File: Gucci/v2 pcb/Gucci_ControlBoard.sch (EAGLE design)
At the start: 70 parts, among them U1 PCA9306_LSSOP, U2 TEENSY_3.6_DIL, U3 MAX4173-SOT-23, U4 MAX4173-SOT-23, U5 LM393-8-SOIC, U6 AP2114H-1.8TRG1, U7 AP2114H-3.3TRG1

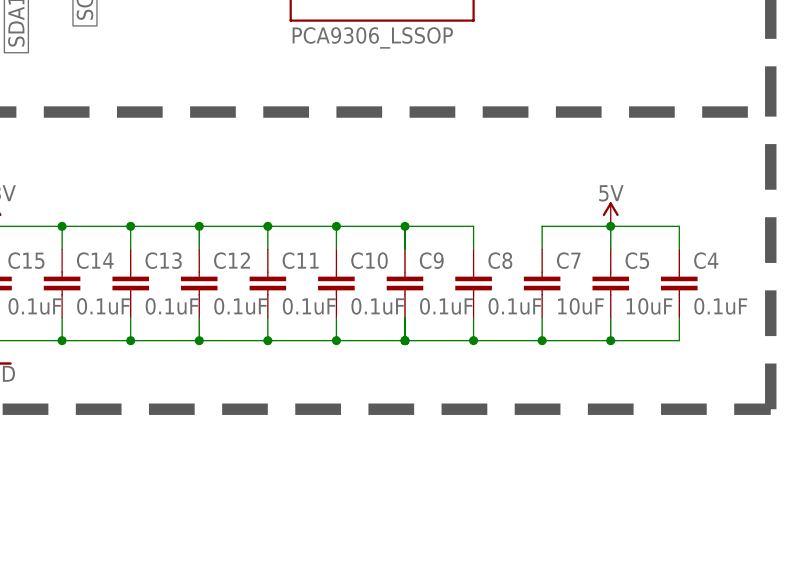
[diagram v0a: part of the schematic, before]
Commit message: board changes per core reviews
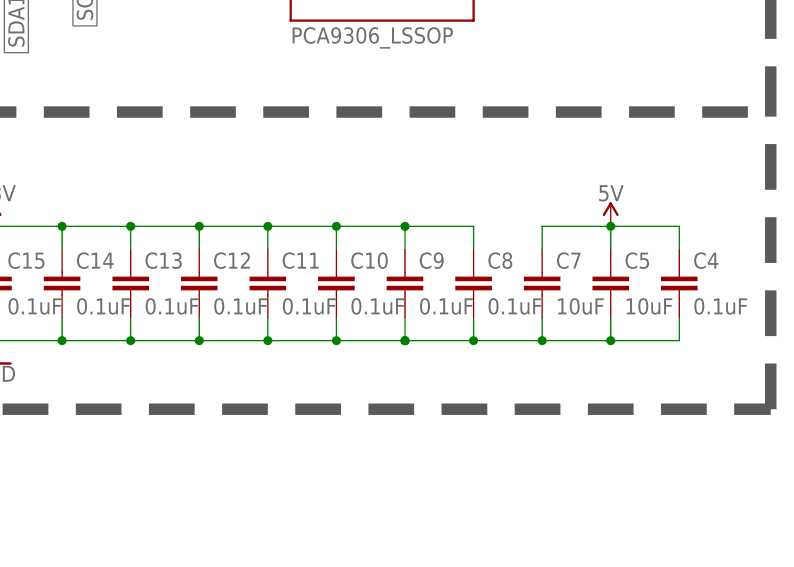
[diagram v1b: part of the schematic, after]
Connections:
- net 3V3 renamed 3.3V
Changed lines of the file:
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@@
 </segment>
 </net>
-<net name="3V3" class="0">
+<net name="3.3V" class="0">
 <segment>
 <pinref part="D2" gate="G$1" pin="A"/>
@@
 <junction x="375.92" y="66.04"/>
 <pinref part="C9" gate="G$1" pin="1"/>
-<wire x1="383.54" y1="66.04" x2="383.54" y2="63.5" width="0.1524" layer="91"/>
 <junction x="383.54" y="66.04"/>
 <pinref part="SUPPLY8" gate="G$1" pin="3.3V"/>
@@
 <junction x="375.92" y="53.34"/>
 <pinref part="C9" gate="G$1" pin="2"/>
-<wire x1="383.54" y1="53.34" x2="383.54" y2="55.88" width="0.1524" layer="91"/>
 <junction x="383.54" y="53.34"/>
 <pinref part="GND26" gate="1" pin="GND"/>
